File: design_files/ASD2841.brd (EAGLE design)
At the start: 22.5 x 29.7 mm, 16 parts, among them J1 DF12-32-DP, J2 DF12-32-DS, J3 SJ-3524-SMT-TR, U1 TS922IDT, U2 MCP4921T-E/MS

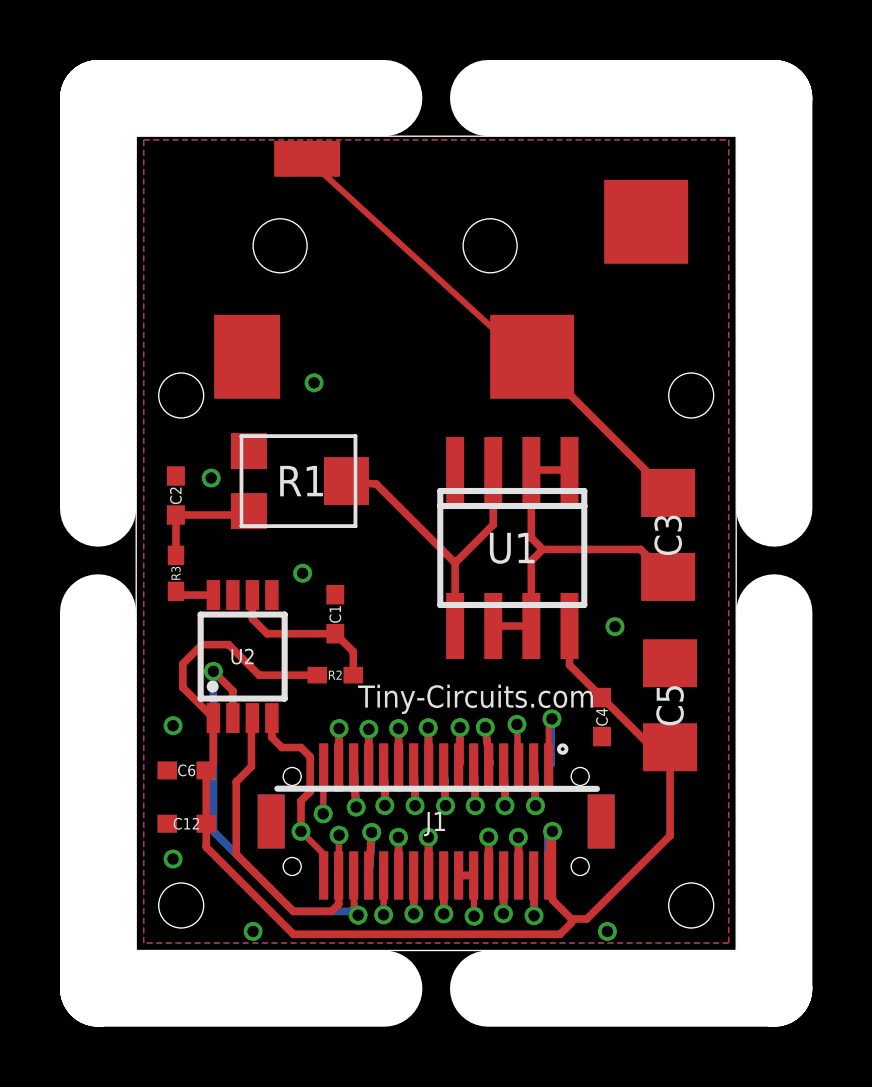
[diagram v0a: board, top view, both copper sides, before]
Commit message: update format
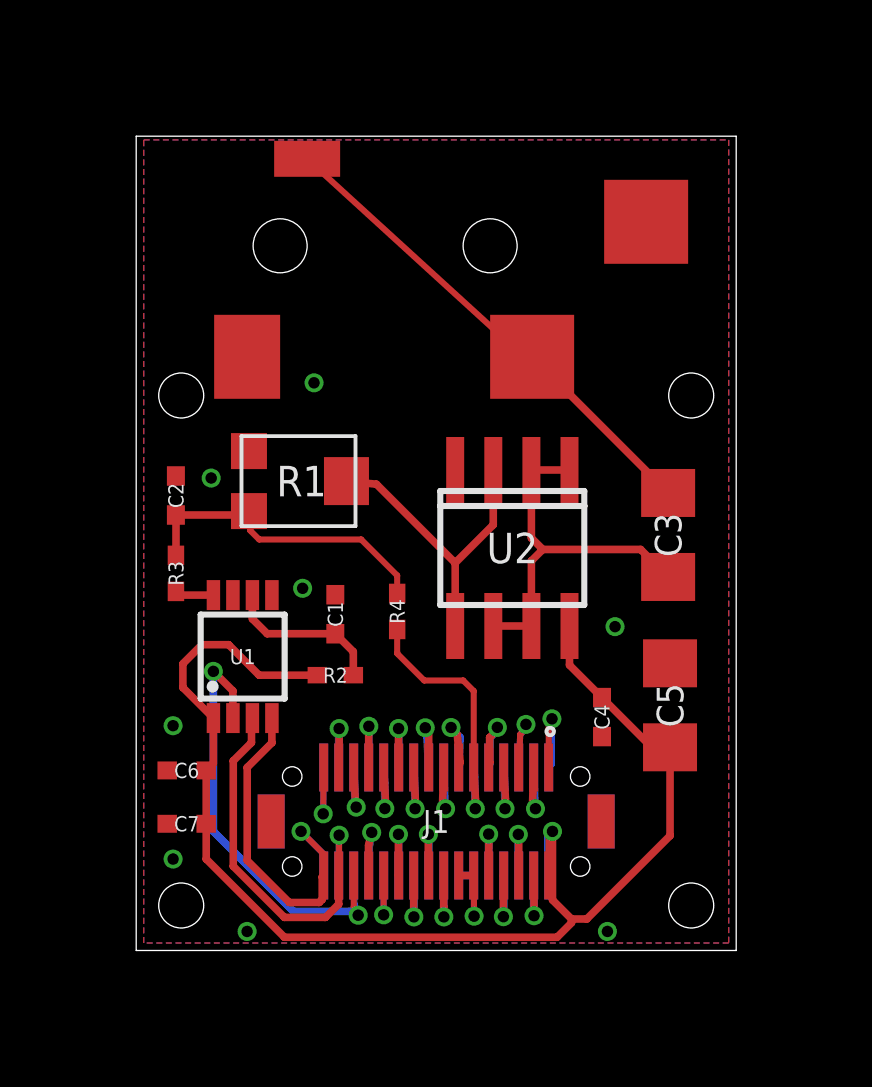
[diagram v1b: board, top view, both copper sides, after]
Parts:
- added R4: 1.00K, tinycircuits:0402
- C7: value 1UF -> 1uF
- U1: value TS922IDT -> MCP4921T-E/MS; device tinycircuits:SO-08 -> tinycircuits:MSOP8
- U2: value MCP4921T-E/MS -> TS922IDT; device tinycircuits:MSOP8 -> tinycircuits:SO-08
- moved U1 9.69 mm to (13.5, 19.8), turned to 0 degrees
- moved U2 9.69 mm to (22.5, 23.4), turned to 180 degrees
- renumbered C12 to C7
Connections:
- net AD0: now also R4.1
- net GND: now also U1.5, U1.7, U2.4; no longer U1.4, U2.5, U2.7
- net IO2: now also U1.2; no longer U2.2
- net IO3: now also U1.3; no longer U2.3
- net IO4: now also U1.4; no longer U2.4
- net N$1: now also U2.3, U2.5; no longer U1.3, U1.5
- net N$2: now also U2.1, U2.2, U2.6, U2.7; no longer U1.1, U1.2, U1.6, U1.7
- net N$3: now also U1.6; no longer U2.6
- net N$4: now also U1.8; no longer U2.8
- net N$9: now also R4.2
- net VCC: now also U1.1, U2.8; no longer U1.8, U2.1
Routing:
- net N$9: track 3.83 -> 10.6 mm
- net AD0: track 2.55 -> 9.17 mm
- net IO4: track 8.37 -> 12.6 mm
- net IO1: track 4.07 -> 2.90 mm
- net IO3: track 12.8 -> 13.3 mm
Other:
- board size 22.5 x 29.7 mm -> 20 x 27.1 mm
- board text added: "5"
- board text added: "ASD2841 - Rev5"
- board text added: "TinyCircuits.com"
- board text removed: "4"
- board text removed: "ASD2841 - Rev4"
- board text removed: "Tiny-Circuits.com"
